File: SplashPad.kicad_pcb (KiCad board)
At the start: 2 copper layers, 100 x 100 mm, 35 parts, among them SW1 SW_Push_45deg, SW10 RotaryEncoder_Switch, SW11 RotaryEncoder_Switch, SW2 SW_Push_45deg, SW3 SW_Push_45deg, SW4 SW_Push_45deg, SW5 SW_Push_45deg, SW6 SW_Push_45deg, SW7 SW_Push_45deg, SW8 SW_Push_45deg, SW9 SW_Push_45deg

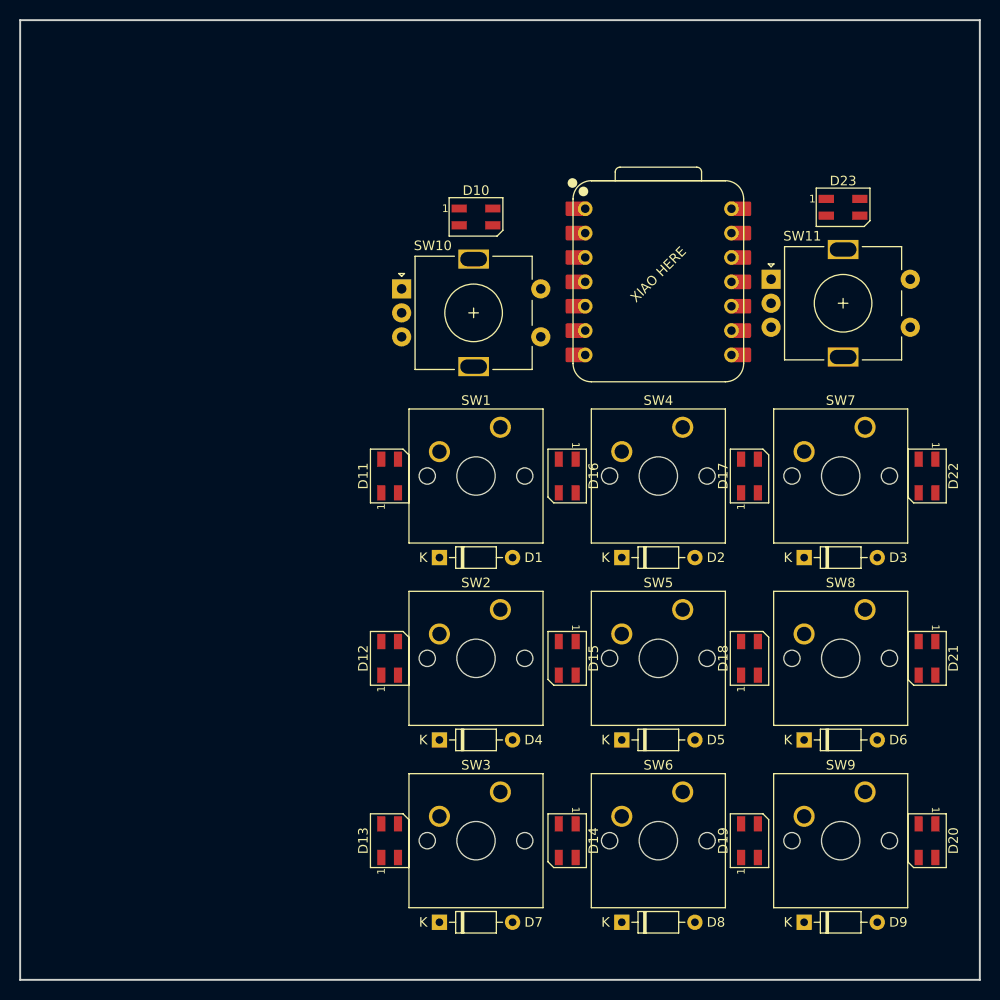
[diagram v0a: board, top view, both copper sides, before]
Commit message: fine tuning
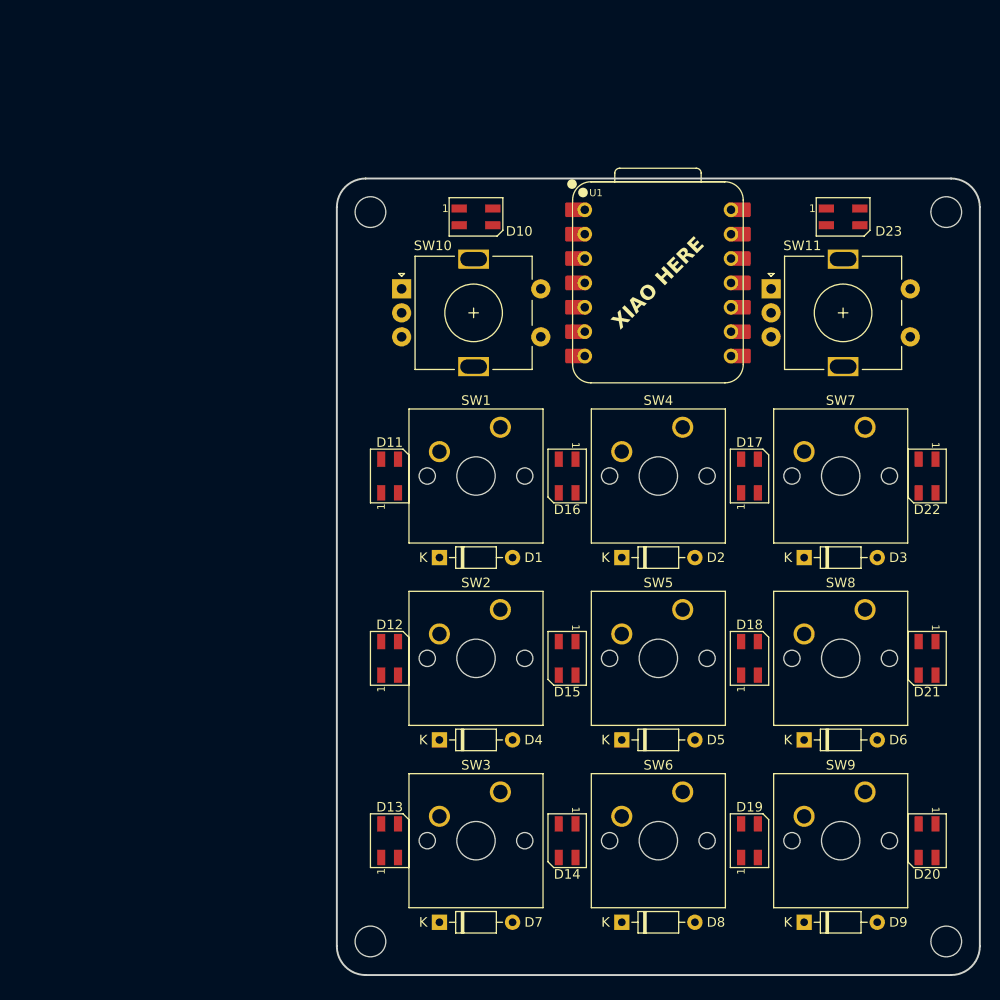
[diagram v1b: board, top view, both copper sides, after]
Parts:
- removed XIAO HERE: XIAO-RP2040-DIP, Seeed Studio XIAO Series Library:XIAO-RP2040-DIP
- added REF**: 3.2mm_M3, MountingHole:MountingHole_3.2mm_M3, F.Cu at (136.5, 146.0)
- added REF**: 3.2mm_M3, MountingHole:MountingHole_3.2mm_M3, F.Cu at (196.5, 146.0)
- added REF**: 3.2mm_M3, MountingHole:MountingHole_3.2mm_M3, F.Cu at (136.5, 70.0)
- added REF**: 3.2mm_M3, MountingHole:MountingHole_3.2mm_M3, F.Cu at (196.5, 70.0)
- added U1: XIAO-RP2040-DIP, Seeed Studio XIAO Series Library:XIAO-RP2040-DIP, F.Cu at (166.5, 77.4)
- moved D23 1.00 mm to (185.8, 70.5)
- moved SW11 1.00 mm to (178.2, 78.0)
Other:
- board size 100 x 100 mm -> 67 x 83 mm
- board text added: "XIAO HERE"
